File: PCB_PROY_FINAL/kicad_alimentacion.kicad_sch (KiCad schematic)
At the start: 10 parts, among them IC3 AP63203WU-7

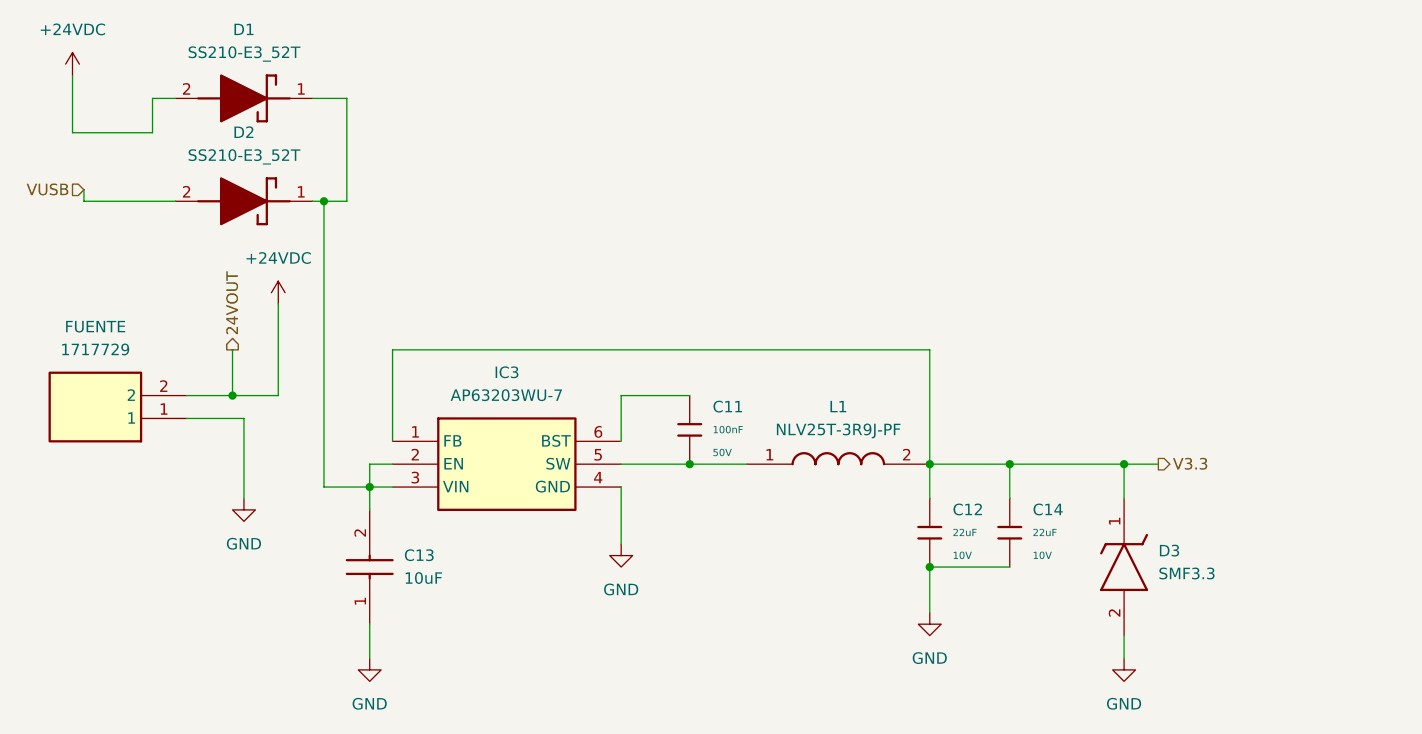
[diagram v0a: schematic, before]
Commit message: Last update pcb
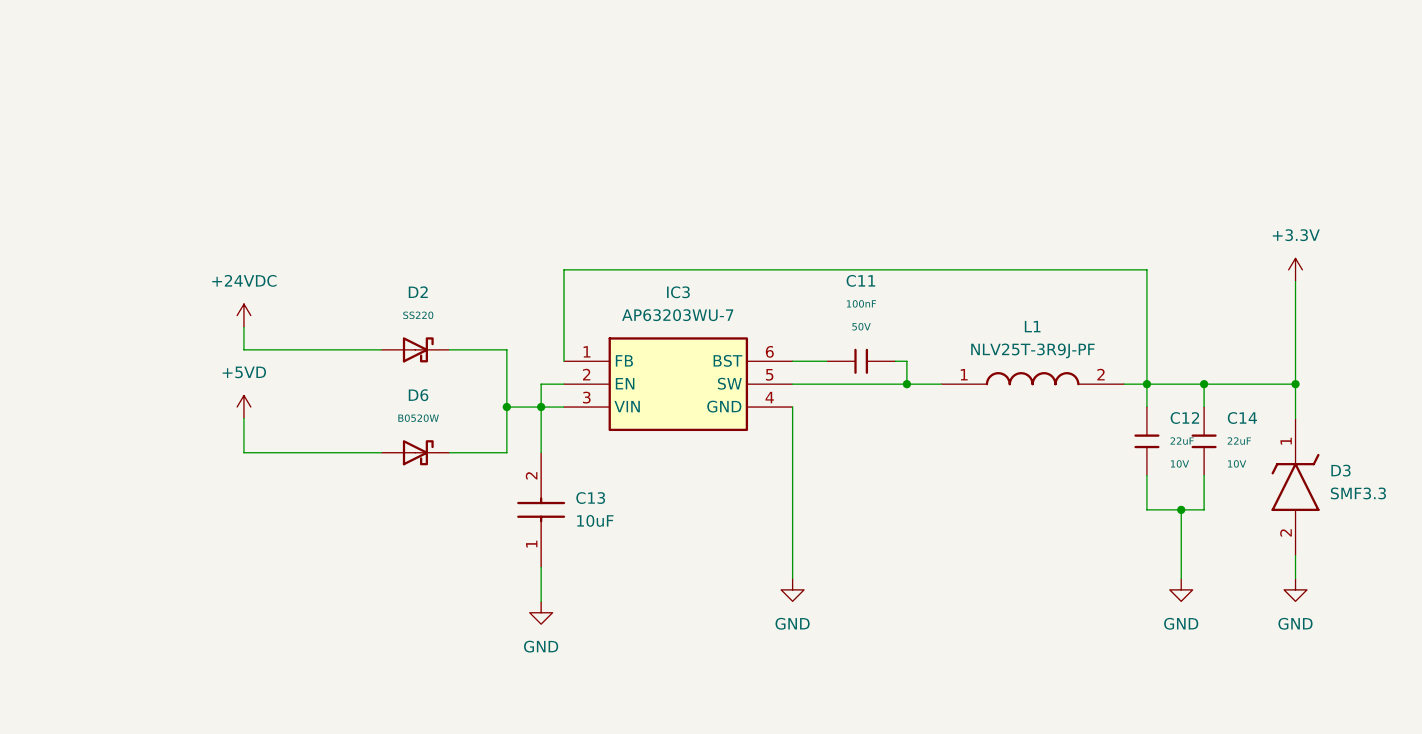
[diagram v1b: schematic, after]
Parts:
- removed D1, D2: SS210-E3_52T, DIONM5436X244N, symbol SamacSys_Parts:SS210-E3_52T
- removed FUENTE: 1717729, 1717729, symbol SamacSys_Parts:1717729
- added D2: SS220, PCM_JLCPCB:D_SMA, symbol PCM_JLCPCB-Diodes:Schottky,SS220
- added D6: B0520W, PCM_JLCPCB:D_SOD-123, symbol PCM_JLCPCB-Diodes:Schottky,B0520W
- C11: LCSC C14663 -> C2392268
- C12, C14: LCSC C5672 -> C2392268
- C13: JLC PART# (none) -> C2803389
- D3: LCSC (none) -> C283866
- IC3: JLCPCB_PART# (none) -> C780769
- L1: LCSC (none) -> C250157
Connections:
- net +24VDC: now also D2.2
- net at C13.2, IC3.2 (EN), IC3.3 (VIN): now also D2.1, D6.1
- net V3.3 renamed +3.3V
- new net +5VD: D6.2
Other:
- moved on the sheet: C11, C12, C13, C14, D3, IC3, L1
